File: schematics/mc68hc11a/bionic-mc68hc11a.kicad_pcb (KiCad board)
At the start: 2 copper layers, 25.4 x 68.6 mm, 8 parts, among them J1 Bionic-P135, J2 Bionic-P245, U1 MC68HC11A0P, U2 11AA010-I/TT

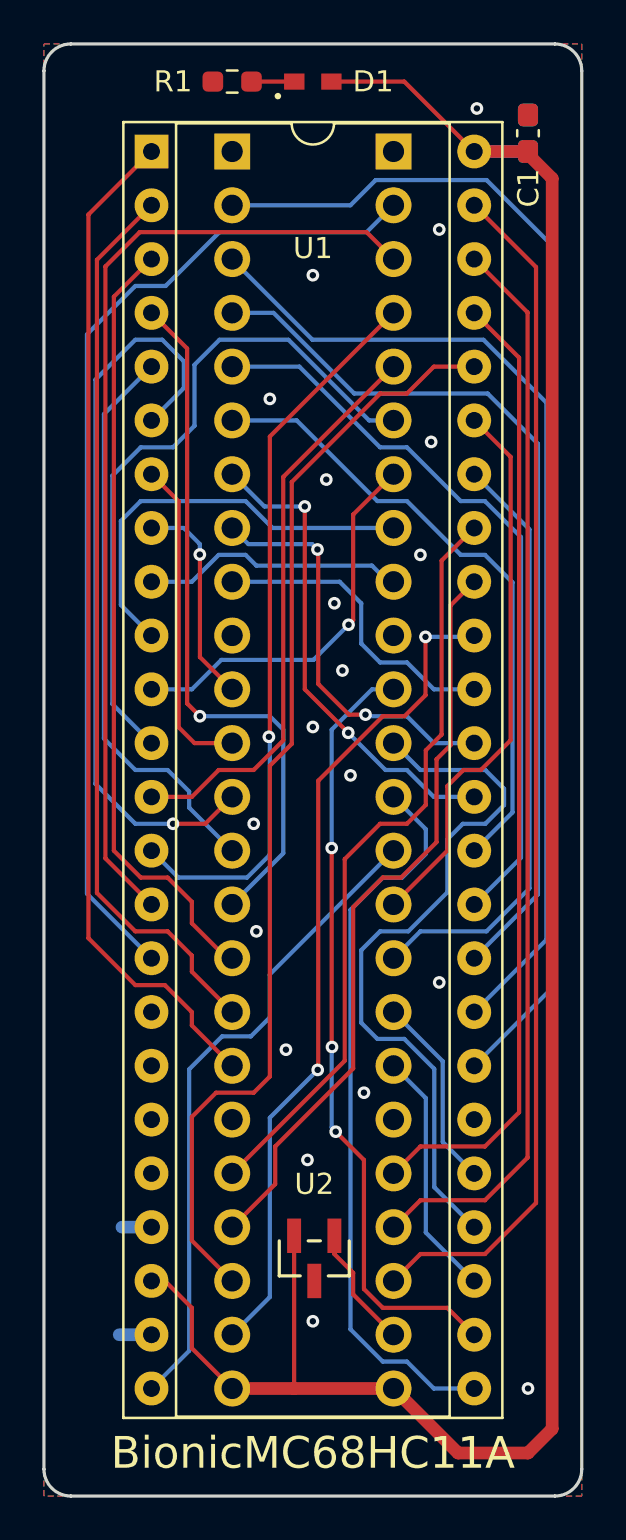
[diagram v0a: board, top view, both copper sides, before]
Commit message: [MC68HC11A] Cleanup schematics
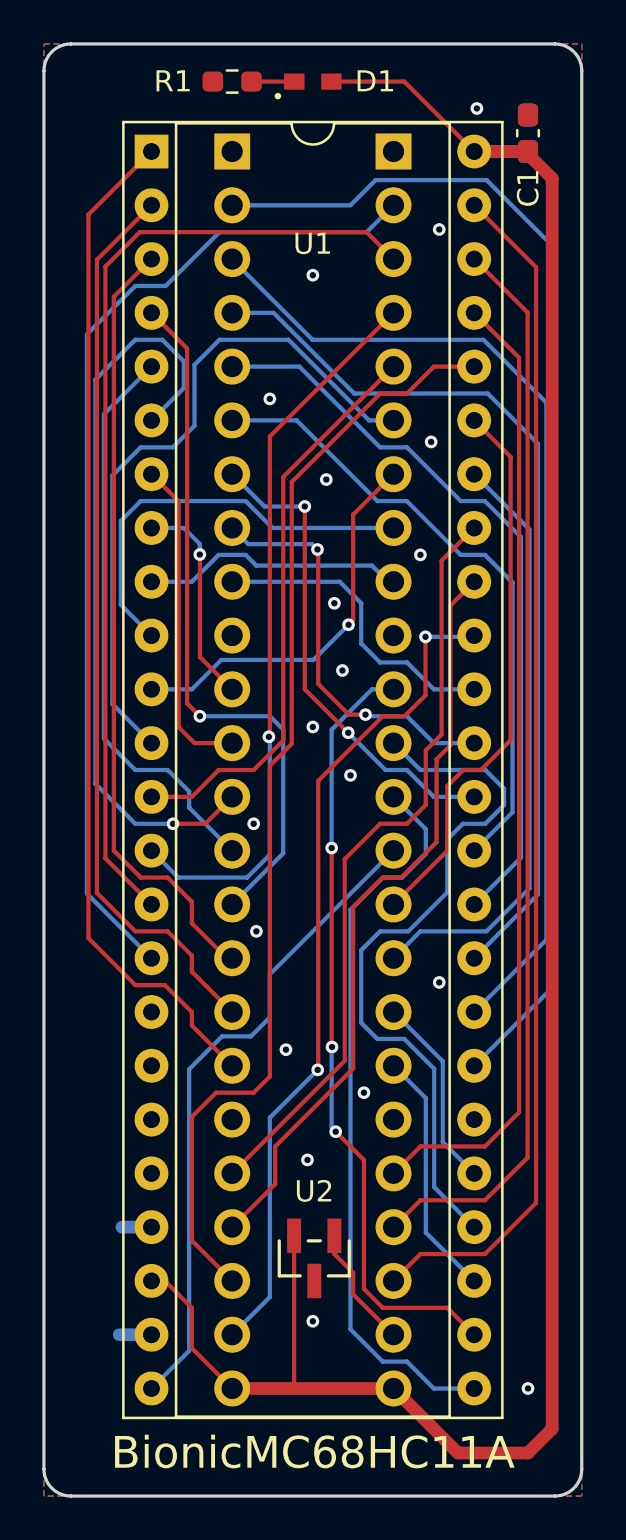
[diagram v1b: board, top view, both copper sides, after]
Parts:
- D1: footprint 0-LocalLibrary:LED_CSL1901UW1_ROM-M -> rhom:LED_CSL1901UW1_ROM-M
- J1: footprint 0-LocalLibrary:Bionic-P135_Vertical -> bionic:Bionic-P135_Vertical
- J2: footprint 0-LocalLibrary:Bionic-P245_Vertical -> bionic:Bionic-P245_Vertical
- U1: footprint 0-LocalLibrary:DIP-48_W15.24mm_Socket -> bionic:DIP-48_W15.24mm_Socket
- U2: footprint 0-LocalLibrary:SOT-23_MC_MCH-M -> microchip:SOT-23_MC_MCH-M
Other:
- rule pad_to_mask_clearance: 0.051 -> 0
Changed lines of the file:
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@@
 			(dielectric_constraints no)
 		)
-		(pad_to_mask_clearance 0.051)
-		(solder_mask_min_width 0.25)
+		(pad_to_mask_clearance 0)
 		(allow_soldermask_bridges_in_footprints no)
 		(aux_axis_origin 101 70)
@@
 		)
 	)
-	(footprint "0-LocalLibrary:DIP-48_W15.24mm_Socket"
+	(footprint "bionic:DIP-48_W15.24mm_Socket"
 		(layer "F.Cu")
 		(at 106.08 75.08)
@@
 		(tags "THT DIP DIL PDIP 2.54mm 15.24mm 600mil Socket")
 		(property "Reference" "U1"
-			(at 7.62 4.572 0)
+			(at 7.62 4.3688 0)
 			(layer "F.SilkS")
 			(effects
@@
 			)
 		)
-		(property "Footprint" "0-LocalLibrary:DIP-48_W15.24mm_Socket"
+		(property "Footprint" "bionic:DIP-48_W15.24mm_Socket"
 			(at 0 0 0)
 			(layer "F.Fab")
@@
 			)
 		)
-		(property "Description" ""
+		(property "Description" "8-bit General Purpose Microprocessor, DIP-48"
 			(at 0 0 0)
 			(layer "F.Fab")
@@
 		)
 	)
-	(footprint "0-LocalLibrary:SOT-23_MC_MCH-M"
+	(footprint "microchip:SOT-23_MC_MCH-M"
 		(layer "F.Cu")
 		(at 113.765999 127.354 180)
-		(tags "11aa010t-i/tt ")
+		(descr "Microchip 11AAxxx-I/TT UNI/O 1Kbit Serial EEPROM")
 		(property "Reference" "U2"
-			(at 0 3.506 0)
+			(at 0 3.1504 0)
 			(unlocked yes)
 			(layer "F.SilkS")
@@
 			)
 		)
-		(property "Footprint" "0-LocalLibrary:SOT-23_MC_MCH-M"
+		(property "Footprint" "microchip:SOT-23_MC_MCH-M"
 			(at 0 0 180)
 			(layer "F.Fab")
@@
 			)
 		)
-		(property "Description" ""
+		(property "Description" "UNI/O Serial EEPROM (1Kbit)"
 			(at 0 0 180)
 			(layer "F.Fab")
@@
 			(pintype "power_in")
 		)
-		(model "${KIPRJMOD}/0-LocalLibrary/SOT-23_MC_MCH.step"
+		(model "${KIPRJMOD}/microchip.pretty/SOT-23_MC_MCH.step"
 			(offset
 				(xyz 0 0 0)
@@
 		)
 	)
-	(footprint "0-LocalLibrary:LED_CSL1901UW1_ROM-M"
+	(footprint "rhom:LED_CSL1901UW1_ROM-M"
 		(layer "F.Cu")
 		(at 113.7 71.778)
@@
 		(tags "CSL1901UW1 ")
 		(property "Reference" "D1"
-			(at 2.8448 0 0)
+			(at 2.9464 0 0)
 			(unlocked yes)
 			(layer "F.SilkS")
@@
 			)
 		)
-		(property "Footprint" "0-LocalLibrary:LED_CSL1901UW1_ROM-M"
+		(property "Footprint" "rhom:LED_CSL1901UW1_ROM-M"
 			(at 0 0 0)
 			(layer "F.Fab")
@@
 			)
 		)
-		(property "Description" ""
+		(property "Description" "Red LED (Low Current Emission, SMD)"
 			(at 0 0 0)
 			(layer "F.Fab")
@@
 			)
 		)
+		(model "${KIPRJMOD}/rhom.pretty/LED_CSL1901UW1_ROM.step"
+			(offset
+				(xyz 0 0 0)
+			)
+			(scale
+				(xyz 1 1 1)
+			)
+			(rotate
+				(xyz 0 0 0)
+			)
+		)
 	)
-	(footprint "0-LocalLibrary:Bionic-P245_Vertical"
+	(footprint "bionic:Bionic-P245_Vertical"
 		(layer "B.Cu")
 		(at 117.51 75.08 180)
@@
 			)
 		)
-		(property "Footprint" "0-LocalLibrary:Bionic-P245_Vertical"
-			(at 0 0 180)
-			(layer "F.Fab")
+		(property "Footprint" "bionic:Bionic-P245_Vertical"
+			(at 0 0 0)
+			(layer "B.Fab")
 			(hide yes)
 			(effects
@@
 					(thickness 0.15)
 				)
+				(justify mirror)
 			)
 		)
 		(property "Datasheet" ""
-			(at 0 0 180)
-			(layer "F.Fab")
+			(at 0 0 0)
+			(layer "B.Fab")
 			(hide yes)
 			(effects
@@
 					(thickness 0.15)
 				)
-			)
-		)
-		(property "Description" ""
-			(at 0 0 180)
-			(layer "F.Fab")
+				(justify mirror)
+			)
+		)
+		(property "Description" "Generic connector, single row, 01x24, script generated (kicad-library-utils/schlib/autogen/connector/)"
+			(at 0 0 0)
+			(layer "B.Fab")
 			(hide yes)
 			(effects
@@
 					(thickness 0.15)
 				)
+				(justify mirror)
 			)
 		)
@@
 		)
 	)
-	(footprint "0-LocalLibrary:Bionic-P135_Vertical"
+	(footprint "bionic:Bionic-P135_Vertical"
 		(layer "B.Cu")
 		(at 109.89 75.08 180)
@@
 			)
 		)
-		(property "Footprint" "0-LocalLibrary:Bionic-P135_Vertical"
-			(at 0 0 180)
-			(layer "F.Fab")
+		(property "Footprint" "bionic:Bionic-P135_Vertical"
+			(at 0 0 0)
+			(layer "B.Fab")
 			(hide yes)
 			(effects
@@
 					(thickness 0.15)
 				)
+				(justify mirror)
 			)
 		)
 		(property "Datasheet" ""
-			(at 0 0 180)
-			(layer "F.Fab")
+			(at 0 0 0)
+			(layer "B.Fab")
 			(hide yes)
 			(effects
@@
 					(thickness 0.15)
 				)
-			)
-		)
-		(property "Description" ""
-			(at 0 0 180)
-			(layer "F.Fab")
+				(justify mirror)
+			)
+		)
+		(property "Description" "Generic connector, single row, 01x24, script generated (kicad-library-utils/schlib/autogen/connector/)"
+			(at 0 0 0)
+			(layer "B.Fab")
 			(hide yes)
 			(effects
@@
 					(thickness 0.15)
 				)
-			)
-		)
+				(justify mirror)
+			)
+		)
